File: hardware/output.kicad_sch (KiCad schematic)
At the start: 10 parts, among them K1 FINDER-30.22, Q2 BSS123, Q3 BSS123

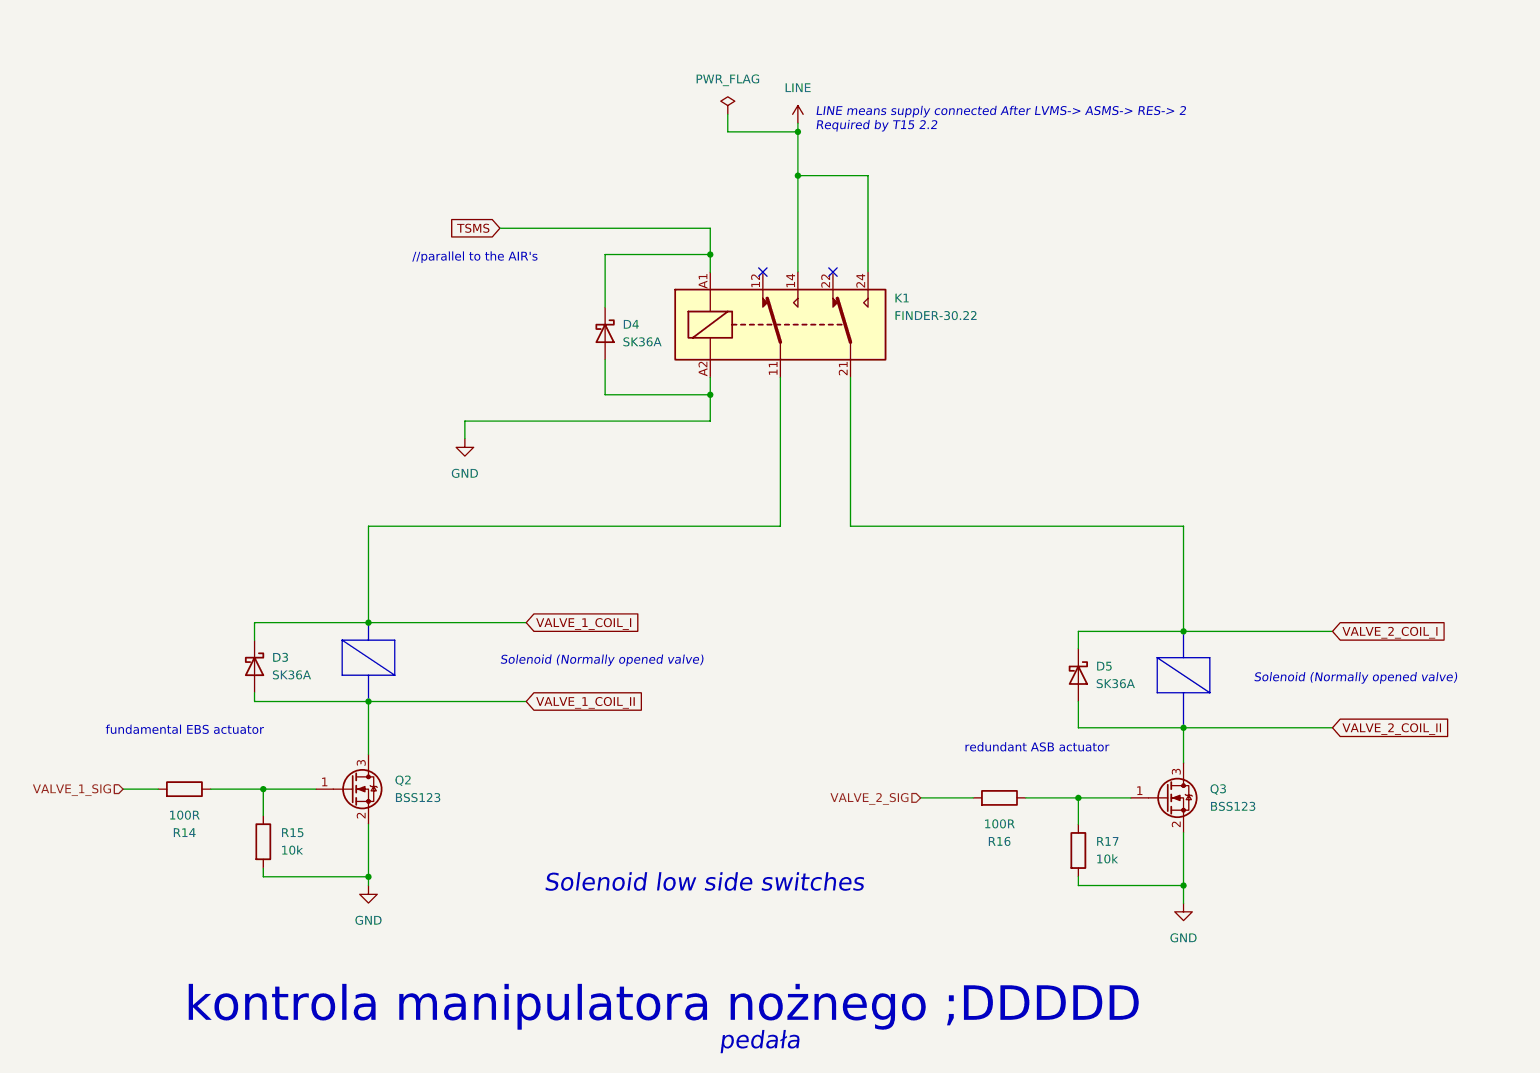
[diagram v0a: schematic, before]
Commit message: changed pcb version
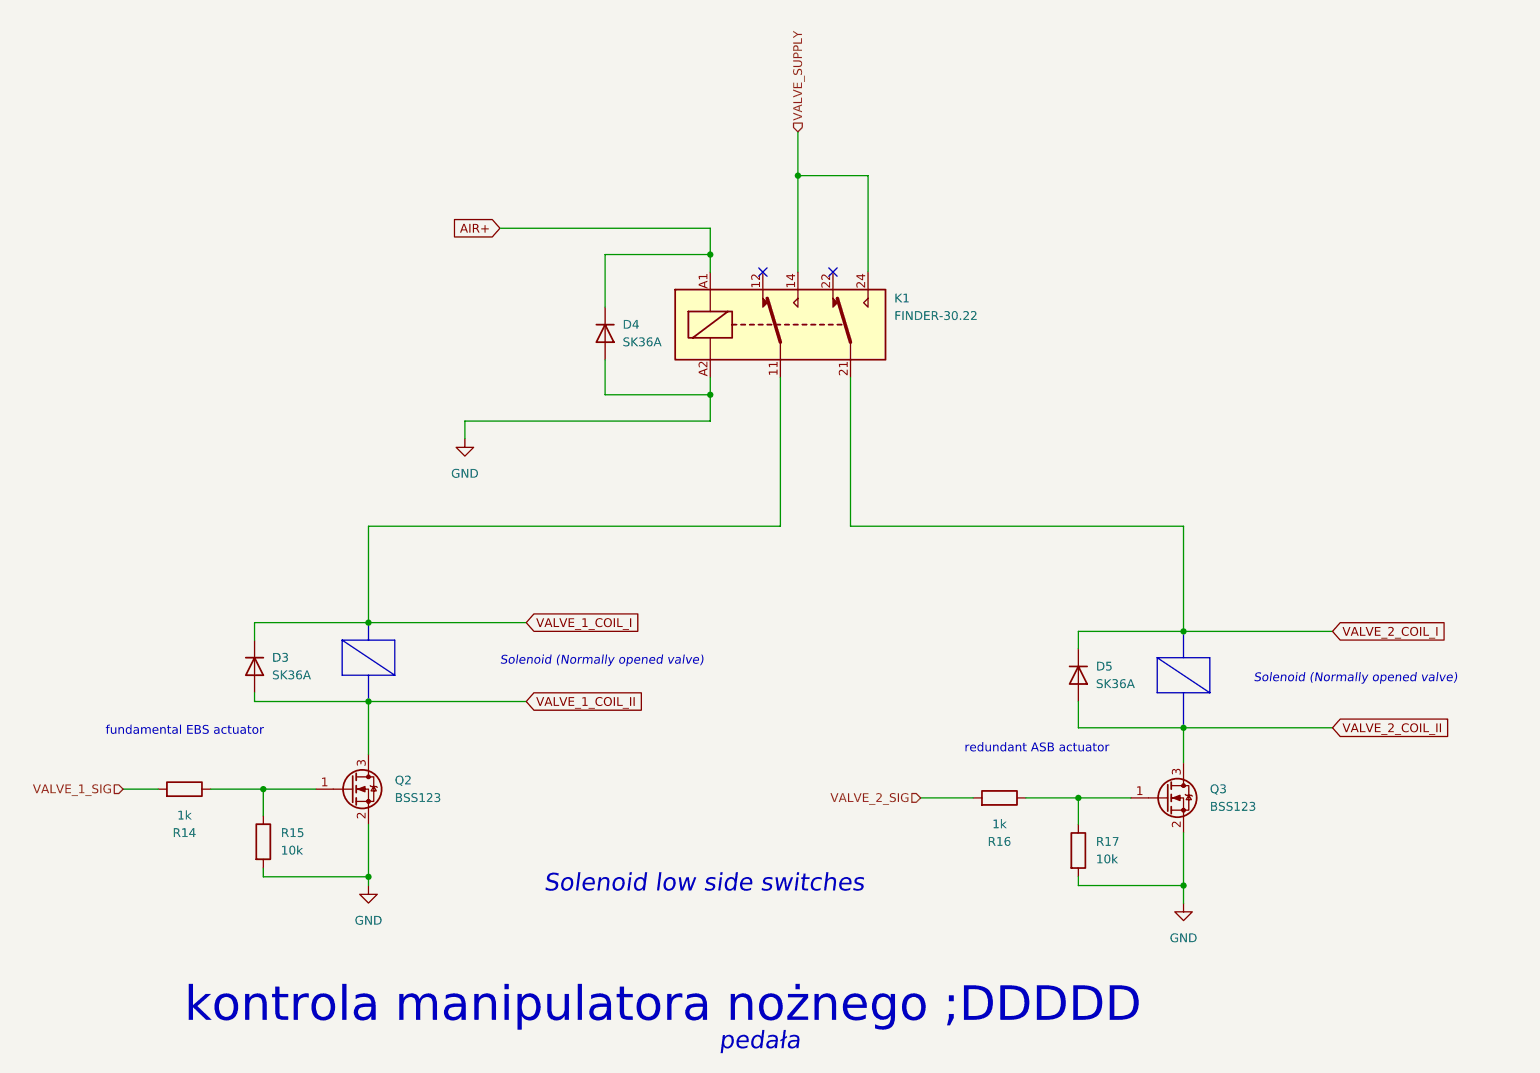
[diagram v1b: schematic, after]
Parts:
- D3, D4, D5: footprint Diode_SMD:D_SMA -> Diode_SMD:D_SMA_Handsoldering; symbol Diode:1N5817 -> Diode:1N5408
- R14, R16: value 100R -> 1k
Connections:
- net LINE renamed VALVE_SUPPLY
- net TSMS renamed AIR+
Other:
- note removed: "//parallel to the AIR's"
- note removed: "LINE means supply connected After LVMS-> ASMS-> RES-> 2 Required by T15 2.2"

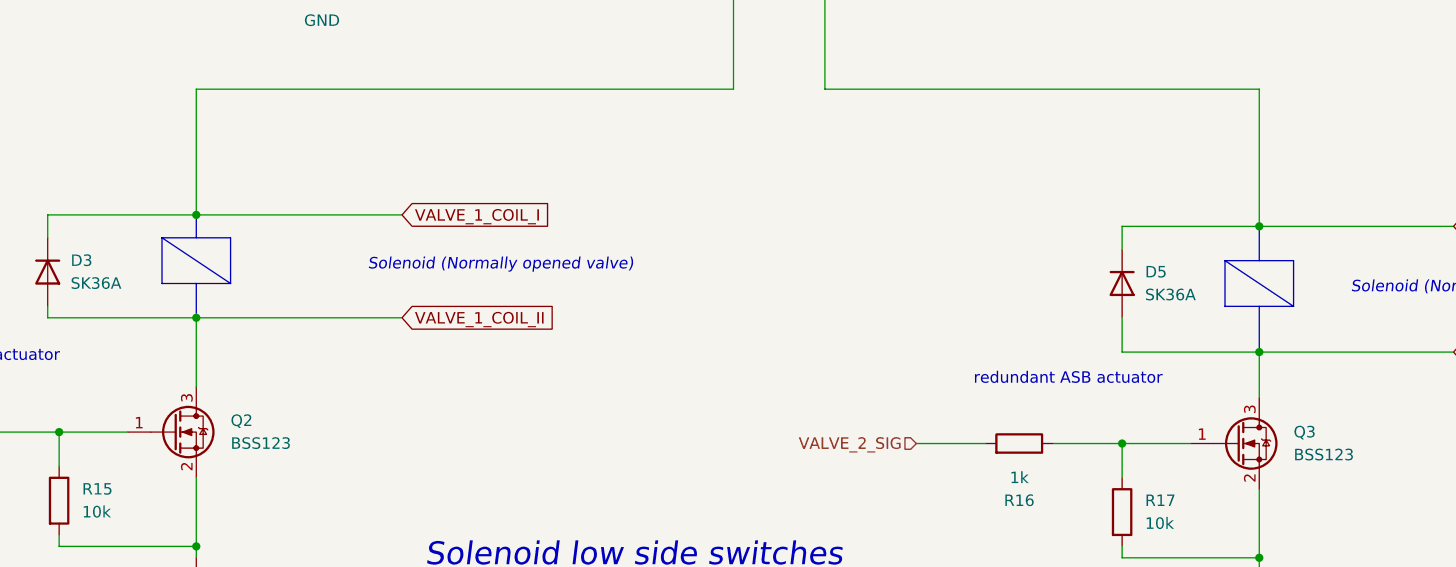
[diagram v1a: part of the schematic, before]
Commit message: uploaded older pcb version
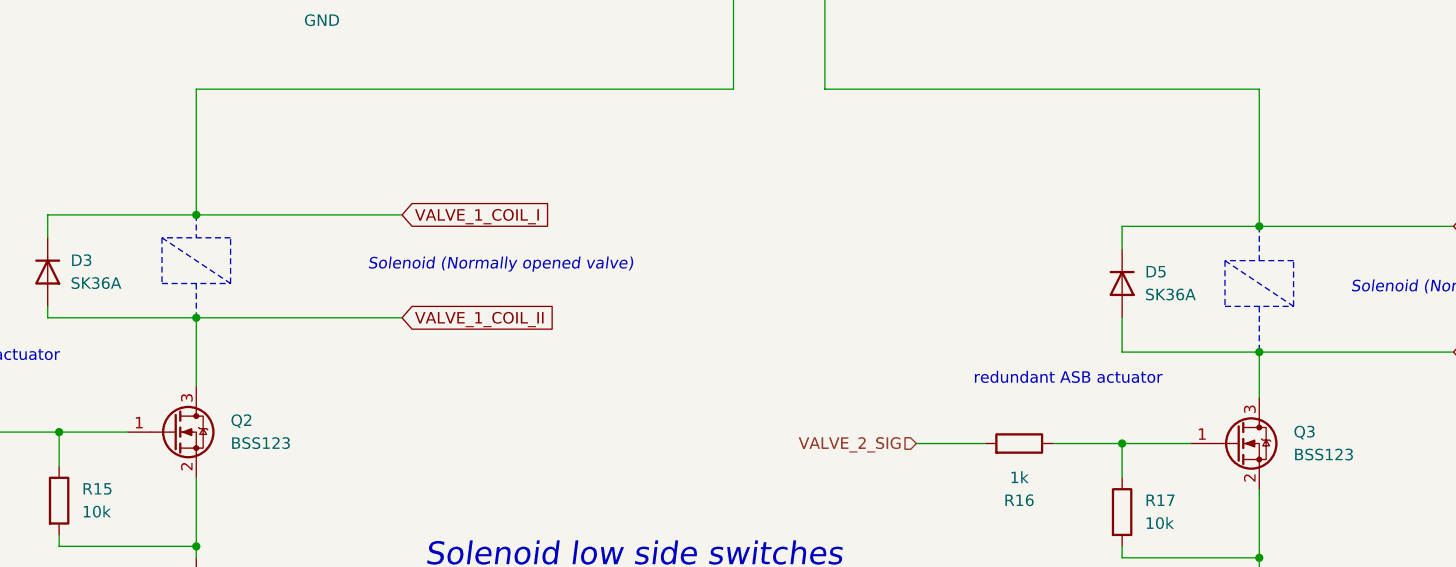
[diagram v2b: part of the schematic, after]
